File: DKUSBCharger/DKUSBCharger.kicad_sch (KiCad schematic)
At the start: 19 parts, among them J1 Conn_01x02, J2 10118192-0002LF, J3 USB_C_Receptacle_USB2.0_16P, J4 USB_A, J5 87583-2010BLF

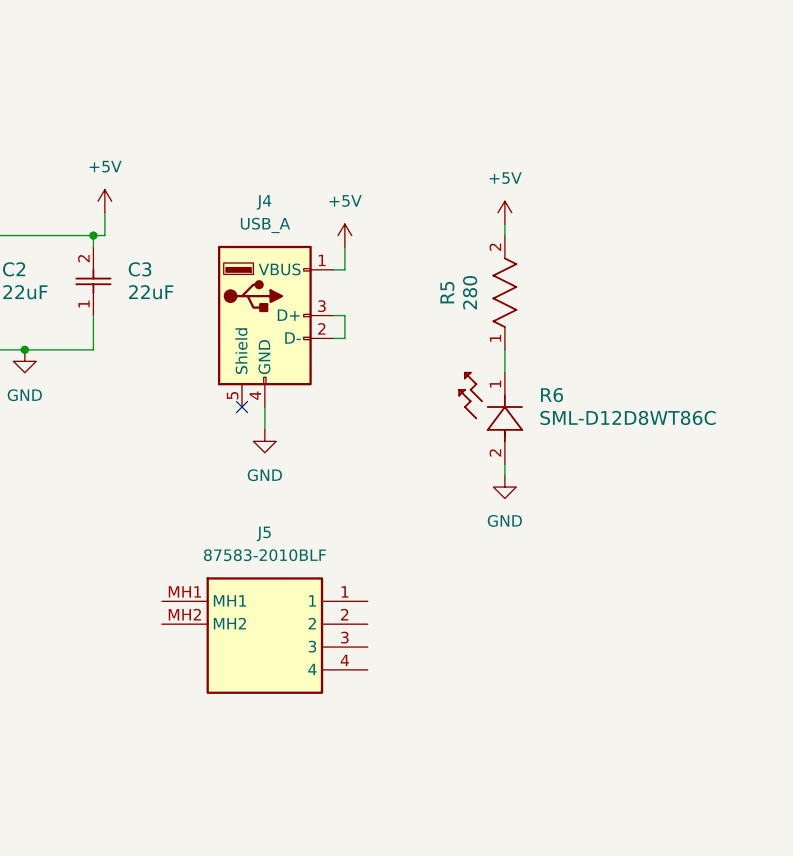
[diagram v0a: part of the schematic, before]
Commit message: Continuing annotations
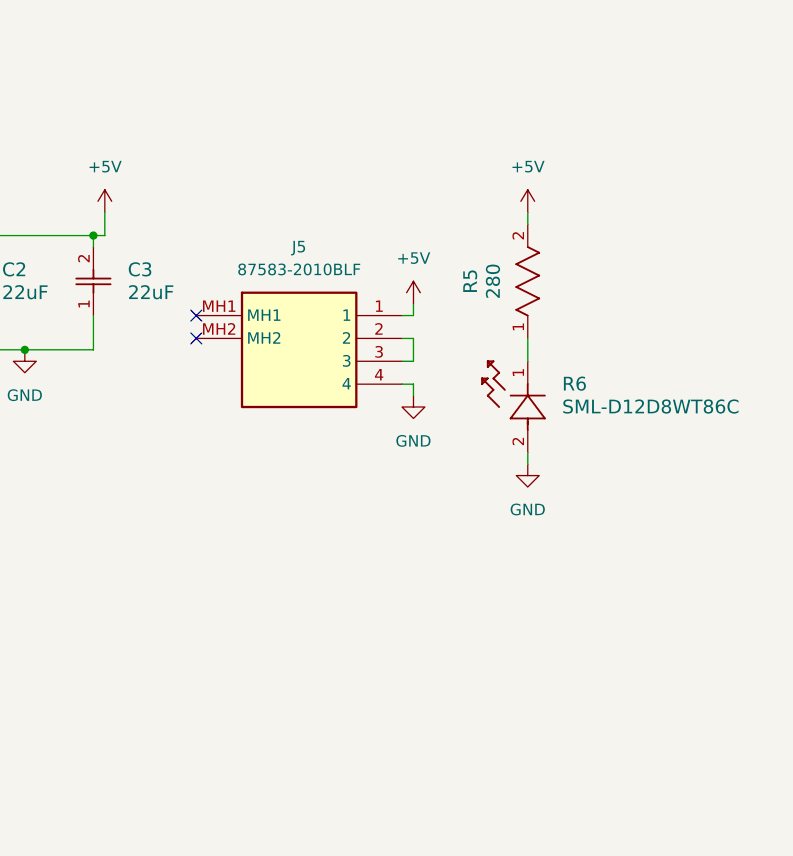
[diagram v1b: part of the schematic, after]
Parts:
- removed J4: USB_A, footprints_USB_Type_A_Receptacle:Conn_USB-87583_AMP, symbol Connector:USB_A
- C1: footprint footprints_10uF_CAP:CAP_CL10_SAM -> USBChargerFootprints:CAP_CL10_SAM
- C2, C3: footprint footprints_22uF_CAP:G-188_MUR -> USBChargerFootprints:G-188_MUR
- J5: footprint 875832010BLF -> USBChargerFootprints:875832010BLF
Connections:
- net +5V: now also J5.1
- net GND: now also J5.4
- net at J5.2: now also J5.3
- no-connect marks 5 -> 6
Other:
- moved on the sheet: J5, R5, R6

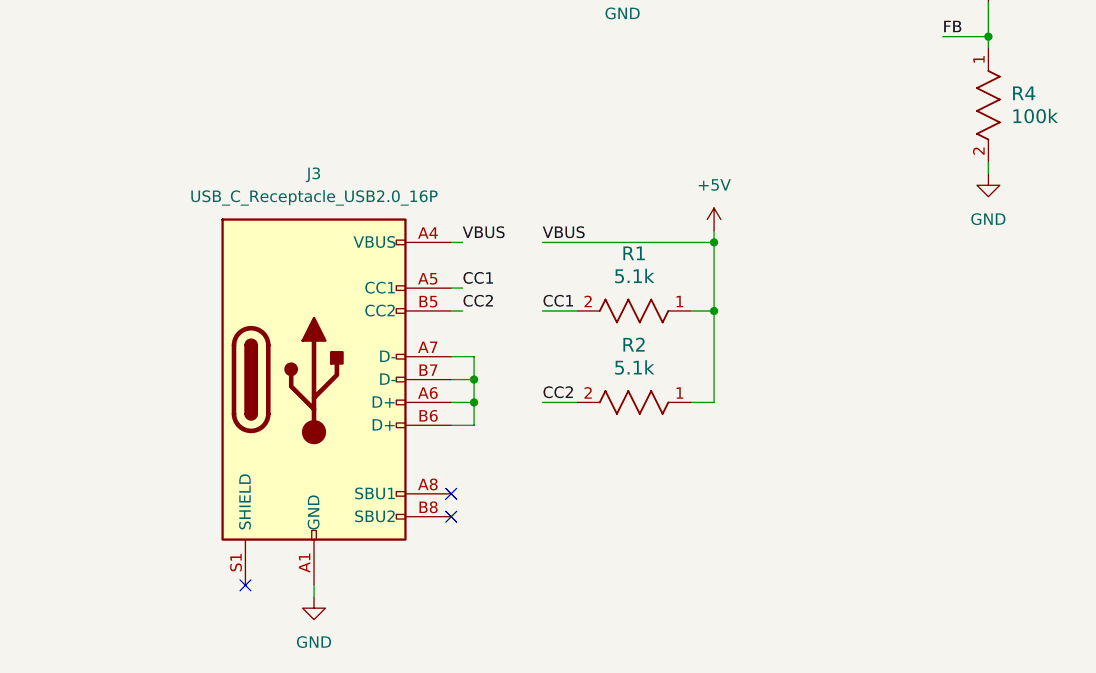
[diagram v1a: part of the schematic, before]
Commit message: Fixed footprints
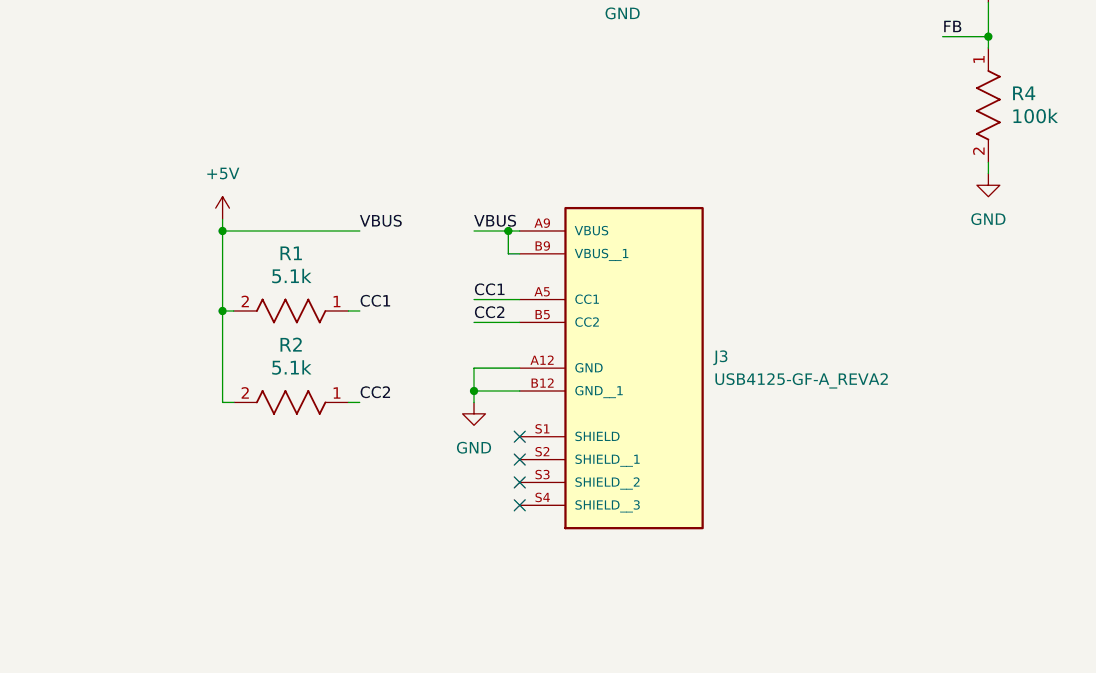
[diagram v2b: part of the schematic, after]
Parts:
- removed J3: USB_C_Receptacle_USB2.0_16P, footprints_USB_Type_C_Receptacle:CONN6_USB4125_GCT, symbol Connector:USB_C_Receptacle_USB2.0_16P
- added J3: USB4125-GF-A_REVA2, USBChargerFootprints:GCT_USB4125-GF-A_REVA2, symbol USBChargerSymbols:USB4125-GF-A_REVA2
- CR1, CR2: footprint footprints_Schottky_60V_3A:SMCDO-214AB_MCC -> USBChargerFootprints:SMCDO-214AB_MCC
- F1: footprint footprints_fuse_2.6A_12V:FUSC4632X205N -> USBChargerFootprints:FUSC4632X205N
- J2: footprint footprints_fuse_2.6A_12V:FUSC4632X205N -> USBChargerFootprints:CONN_10118192-0002LF_AMP
- L1: footprint Inductor_1uF:INDC2012X80N -> USBChargerFootprints:INDC2012X80N
- R1, R2: footprint footprints_resistor_5.1k:RC0603N_YAG-M -> USBChargerFootprints:RC0603N_YAG
- R3: footprint Resistor_732k:RC0603N_PAN -> USBChargerFootprints:RC0603N_PAN
- R4: footprint footprints_resistor_100k:RC0603N_PAN -> USBChargerFootprints:RC0603N_PAN_100k
- R5: footprint RR0816P_2800_D_44A:RESC1608X50N -> USBChargerFootprints:RESC1608X50N
- R6: footprint footprints_LED_orange:LED_SMLD12_ROM -> USBChargerFootprints:LED_SMLD12_ROM
- U1: footprint footprints_regulator_boost_3A_ADJ:DRL0006A -> USBChargerFootprints:DRL0006A
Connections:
- net +5V: now also R1.2, R2.2, J3.A9 (VBUS), J3.B9 (VBUS__1); no longer R1.1, R2.1
- net CC1: now also R1.1, J3.A5 (CC1); no longer R1.2
- net CC2: now also R2.1, J3.B5 (CC2); no longer R2.2
- net GND: now also J3.A12 (GND), J3.B12 (GND__1)
- no-connect marks 6 -> 7
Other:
- moved on the sheet: R1, R2
